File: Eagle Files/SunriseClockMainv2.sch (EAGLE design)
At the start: 18 parts

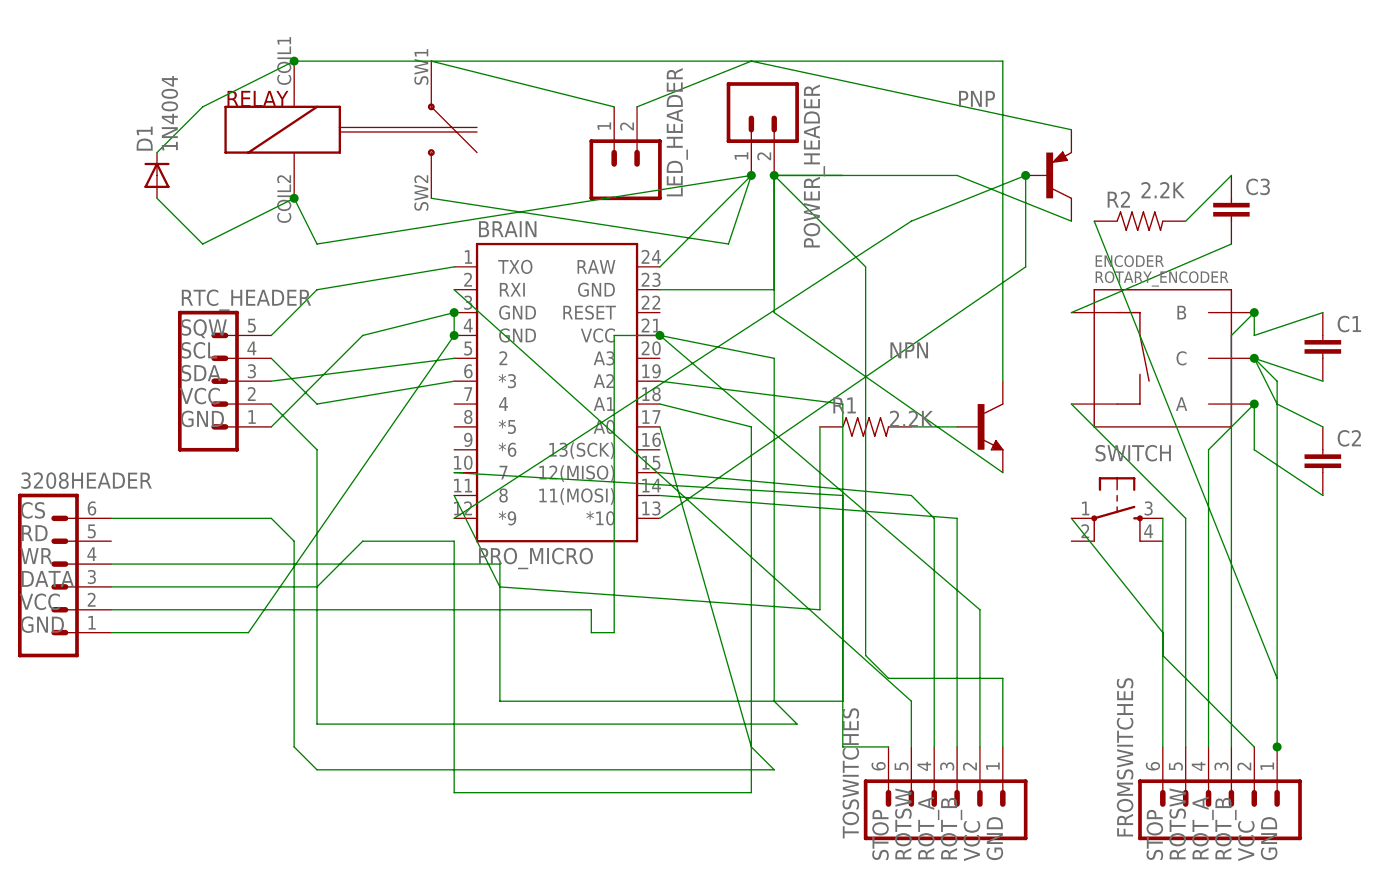
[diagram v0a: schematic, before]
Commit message: V3.1
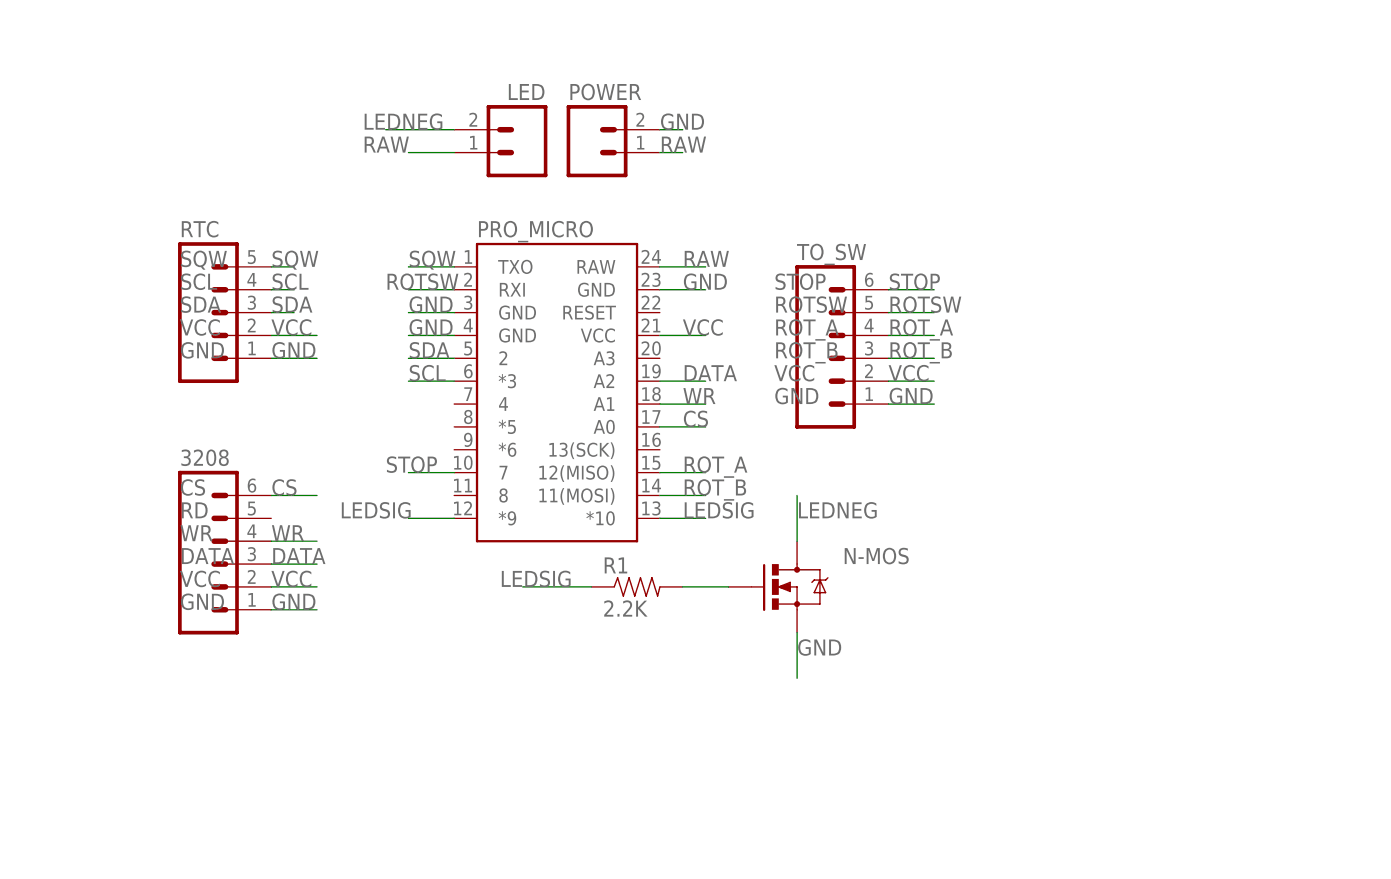
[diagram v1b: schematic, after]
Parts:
- removed 3208HEADER, FROMSWITCHES, TOSWITCHES: (no value), SparkFun-Connectors:M06LOCK
- removed C1, C2, C3: (no value), SparkFun-Capacitors:CAPEZ
- removed D1: 1N4004, diode:1N4004
- removed ENCODER: ROTARY_ENCODER, SparkFun-Electromechanical:ROTARTY_ENCODER
- removed LED_HEADER: (no value), SparkFun-Connectors:M02LOCK
- removed NPN: (no value), transistor:-NPN-TO126V
- removed PNP: (no value), transistor:-PNP-TO126V
- removed POWER_HEADER: (no value), SparkFun-Connectors:M025MM
- removed R2: (no value), SparkFun-Resistors:RESISTORPTH-1/4W
- removed RELAY: RELAY, haller-relais:BV-1254
- removed RTC_HEADER: (no value), SparkFun-Connectors:M05LOCK
- removed SWITCH: (no value), SparkFun-Retired:TAC_SWITCHPTH
- added 3208, TO_SW: (no value), SparkFun-Connectors:M06LOCK
- added LED: (no value), SparkFun-Connectors:M02LOCK
- added N-MOS: MOSFET-NCHANNELFQP30N06L, SparkFun-DiscreteSemi:MOSFET-NCHANNELFQP30N06L
- added POWER: (no value), SparkFun-Connectors:M025MM
- added RTC: (no value), SparkFun-Connectors:M05LOCK
- PRO_MICRO: value PRO_MICRO -> ARDUINO_PRO_MICRO
- R1: value (none) -> 2.2K; R1 2.2K -> (none)
- renumbered BRAIN to PRO_MICRO
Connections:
- removed net N$10: NPN.E, PNP.C, POWER_HEADER.2, PRO_MICRO.GND@2, TOSWITCHES.1
- removed net N$11: C2.2, ENCODER.A, FROMSWITCHES.4
- removed net N$12: C3.1, R2.2
- removed net N$13: C3.2, ENCODER.SW+
- removed net N$14: PRO_MICRO.RXI, TOSWITCHES.5
- removed net N$15: PRO_MICRO.7, TOSWITCHES.6
- removed net N$16: FROMSWITCHES.2, SWITCH.3
- removed net N$17: PRO_MICRO.TXO, RTC_HEADER.5
- removed net N$18: C1.2, C2.1, ENCODER.C, FROMSWITCHES.1, R2.1
- removed net N$19: 3208HEADER.2, PRO_MICRO.VCC, RTC_HEADER.2, TOSWITCHES.2
- removed net N$2: LED_HEADER.1, RELAY.SW1
- removed net N$20: PRO_MICRO.*3, RTC_HEADER.4
- removed net N$21: PRO_MICRO.2, RTC_HEADER.3
- removed net N$22: ENCODER.SW-, FROMSWITCHES.5
- removed net N$23: 3208HEADER.1, PRO_MICRO.GND, PRO_MICRO.GND@1, RTC_HEADER.1
- removed net N$24: 3208HEADER.6, PRO_MICRO.A0
- removed net N$25: 3208HEADER.4, PRO_MICRO.A1
- removed net N$26: 3208HEADER.3, PRO_MICRO.A2
- removed net N$27: PRO_MICRO.12(MISO), TOSWITCHES.4
- removed net N$28: PRO_MICRO.11(MOSI), TOSWITCHES.3
- removed net N$29: D1.C, NPN.C, RELAY.COIL1
- removed net N$3: LED_HEADER.2, PNP.E
- removed net N$4: FROMSWITCHES.6, SWITCH.1
- removed net N$5: PNP.B, PRO_MICRO.*10, PRO_MICRO.*9
- removed net N$7: PRO_MICRO.8, R1.1
- removed net N$8: NPN.B, R1.2
- removed net N$9: C1.1, ENCODER.B, FROMSWITCHES.3
- new net CS: 3208.6, PRO_MICRO.A0
- new net DATA: 3208.3, PRO_MICRO.A2
- new net GND: 3208.1, N-MOS.S, POWER.2, PRO_MICRO.GND, PRO_MICRO.GND@1, PRO_MICRO.GND@2, RTC.1, TO_SW.1
- new net LEDNEG: LED.2, N-MOS.D
- new net LEDSIG: PRO_MICRO.*10, PRO_MICRO.*9, R1.1
- new net RAW: LED.1, POWER.1, PRO_MICRO.RAW
- new net ROTSW: PRO_MICRO.RXI, TO_SW.5
- new net ROT_A: PRO_MICRO.12(MISO), TO_SW.4
- new net ROT_B: PRO_MICRO.11(MOSI), TO_SW.3
- new net SCL: PRO_MICRO.*3, RTC.4
- new net SDA: PRO_MICRO.2, RTC.3
- new net SQW: PRO_MICRO.TXO, RTC.5
- new net STOP: PRO_MICRO.7, TO_SW.6
- new net VCC: 3208.2, PRO_MICRO.VCC, RTC.2, TO_SW.2
- new net WR: 3208.4, PRO_MICRO.A1
- net N$1: now also N-MOS.G, R1.2; no longer D1.A, POWER_HEADER.1, PRO_MICRO.RAW, RELAY.COIL2, RELAY.SW2
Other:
- moved on the sheet: R1
